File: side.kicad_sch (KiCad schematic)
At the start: 74 parts, among them J1 Conn_01x02_Pin, J2 HRO_TYPE-C-31-M-14, J3 Battery, J9 TC2030_SWD, Q2 2N7002, SW1 PWR, SW2 RST, U1 SRV05-4, U10 MAX17048, U3 BQ24075, U8 nRF52840_moko_mk08

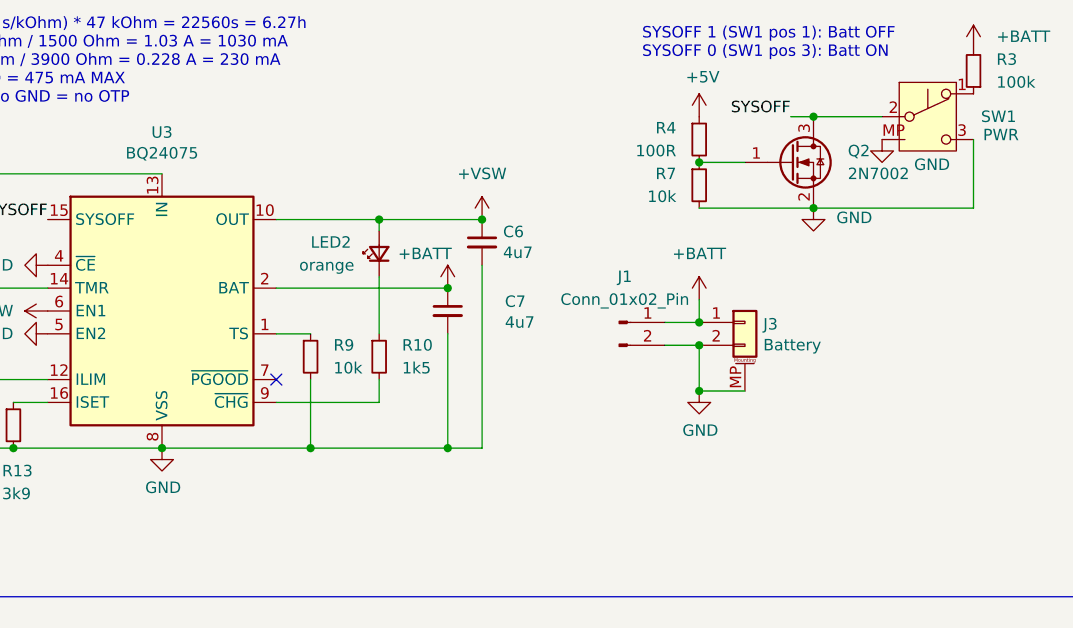
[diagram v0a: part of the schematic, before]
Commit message: post crash
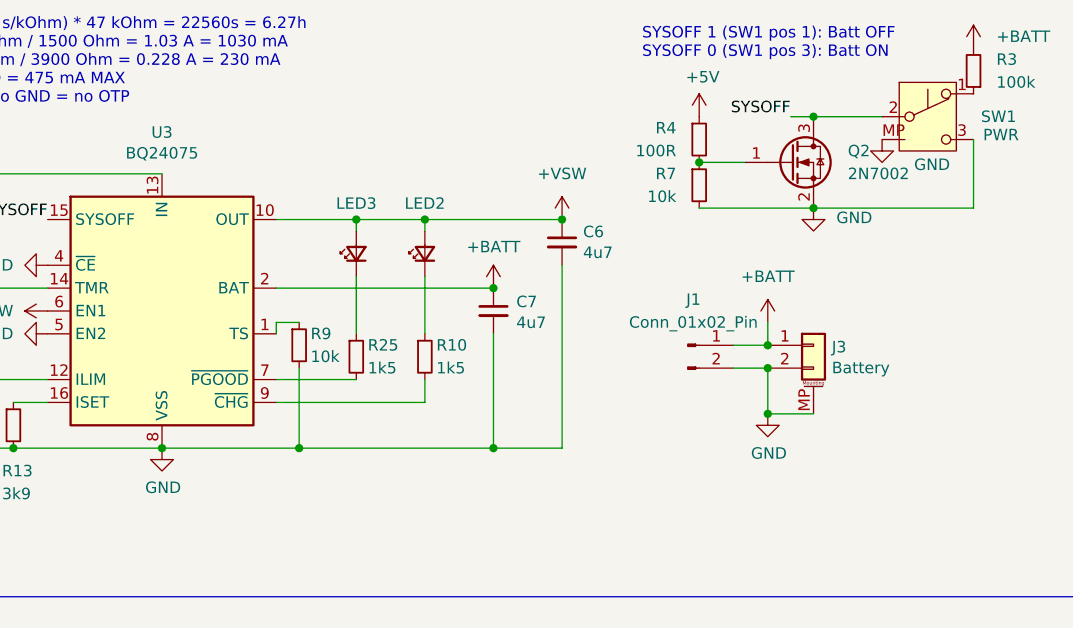
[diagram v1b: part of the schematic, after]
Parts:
- added LED3: LT VH9G-Q2OO-25-1, LED_SMD:LED_0402_1005Metric, symbol Device:LED_Small
- added R25: 1k5, Resistor_SMD:R_0402_1005Metric, symbol Device:R_Small
- LED2: value orange -> LW QH8G-Q2OO-3K5L-1
- U8: now left out of the parts list
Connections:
- net +VSW: now also LED3.2 (A)
- net at U3.7 (~{PGOOD}): now also R25.2
- new net: LED3.1 (K), R25.1
- no-connect marks 48 -> 47
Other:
- moved on the sheet: C6, C7, J1, J3, LED2, R10, R9

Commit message: update VQFN-16-1EP_3x3mm_P0.5mm_EP1.6x1.6mm footprint
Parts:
- U3: footprint Package_DFN_QFN:VQFN-16-1EP_3x3mm_P0.5mm_EP1.6x1.6mm -> kigraz:VQFN-16-1EP_3x3mm_P0.5mm_EP1.6x1.6mm
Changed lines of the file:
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@@
 			)
 		)
-		(property "Footprint" "Package_DFN_QFN:VQFN-16-1EP_3x3mm_P0.5mm_EP1.6x1.6mm"
+		(property "Footprint" "kigraz:VQFN-16-1EP_3x3mm_P0.5mm_EP1.6x1.6mm"
 			(at 179.07 68.58 0)
 			(hide yes)
